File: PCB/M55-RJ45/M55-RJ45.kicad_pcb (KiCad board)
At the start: 2 copper layers, 45.2 x 31 mm, 6 parts, among them J1 RJ45, J2 M55 Archer male, J3 RJ45, J4 M55 Archer female

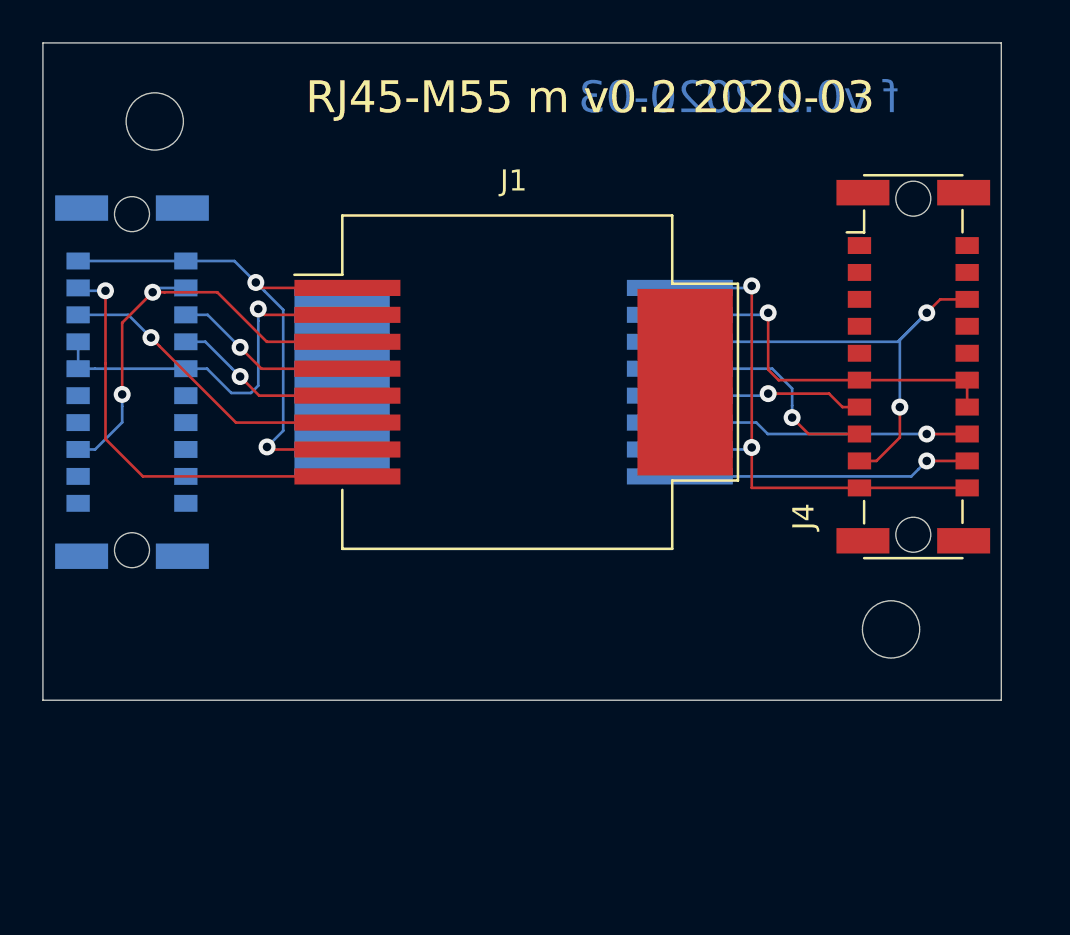
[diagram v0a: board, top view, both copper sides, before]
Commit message: two-sided draft
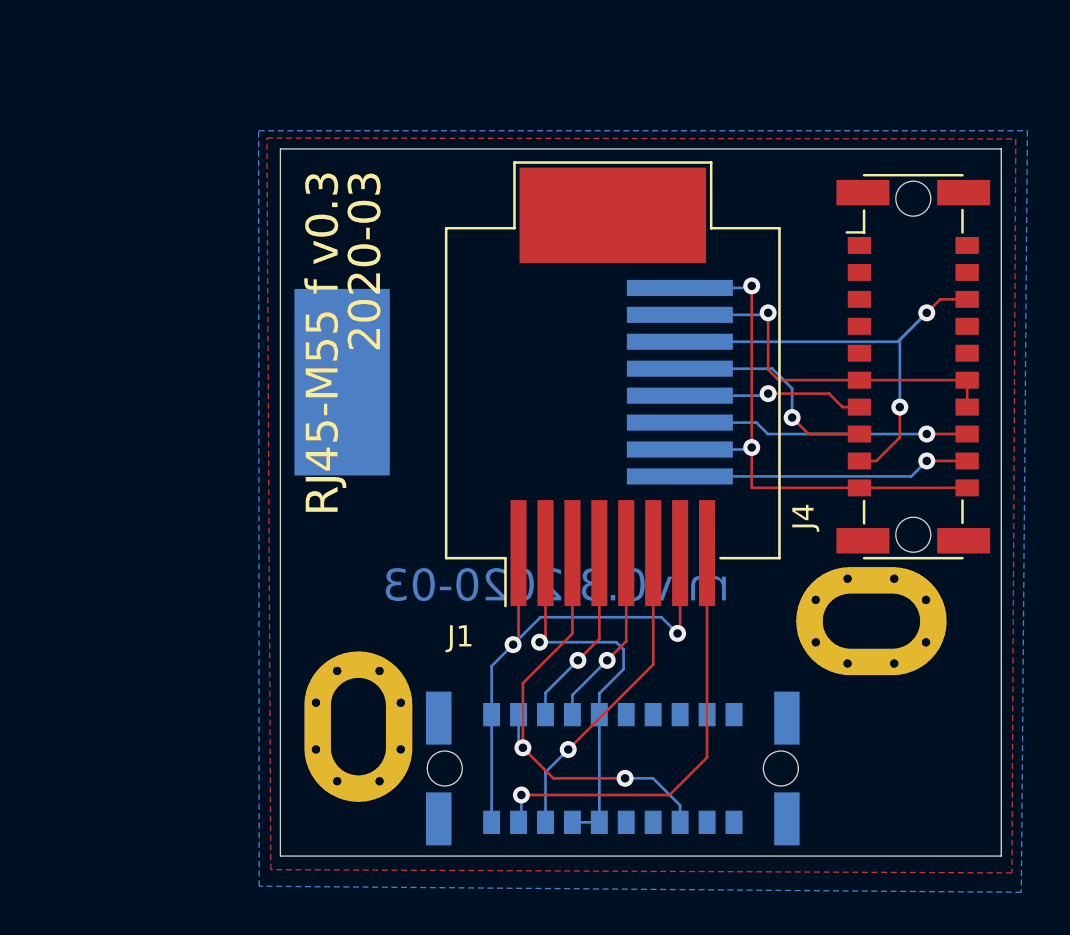
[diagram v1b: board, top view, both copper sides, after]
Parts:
- removed the REF** at (68.8, 140.7)
- removed the REF** at (34.1, 116.7)
- added REF**: MountingHole_2.5x4mm_Pad_VIA, connectors:Mount_via, F.Cu at (43.7, 145.2)
- added REF**: MountingHole_2.5x4mm_Pad_VIA, connectors:Mount_via, F.Cu at (67.8, 140.3)
- moved J2 29.1 mm to (55.7, 147.2), turned to 180 degrees
- moved J1 4.68 mm to (55.7, 129.2), turned to 90 degrees
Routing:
- added copper zone on B.Cu, net (none)
- added copper zone on F.Cu, net (none)
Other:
- board size 45.2 x 31 mm -> 34 x 33.3 mm
- rule trace_min: 0.2 -> 0.127
- board text added: "2020-03"
- board text added: "RJ45-M55 f v0.3"
- board text added: "f"
- board text added: "m"
- board text added: "m v0.3 2020-03"
- board text removed: "RJ45-M55 m v0.2 2020-03"
- board text removed: "f v0.2 2020-03"
